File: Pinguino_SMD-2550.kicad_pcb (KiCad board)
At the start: 2 copper layers, 25.4 x 25.4 mm, 18 parts, among them P1 USB_OTG, P2 CONN_01X08, P3 CONN_01X02, P4 CONN_01X10, SW1 SW Reset, Y1 20Mhz

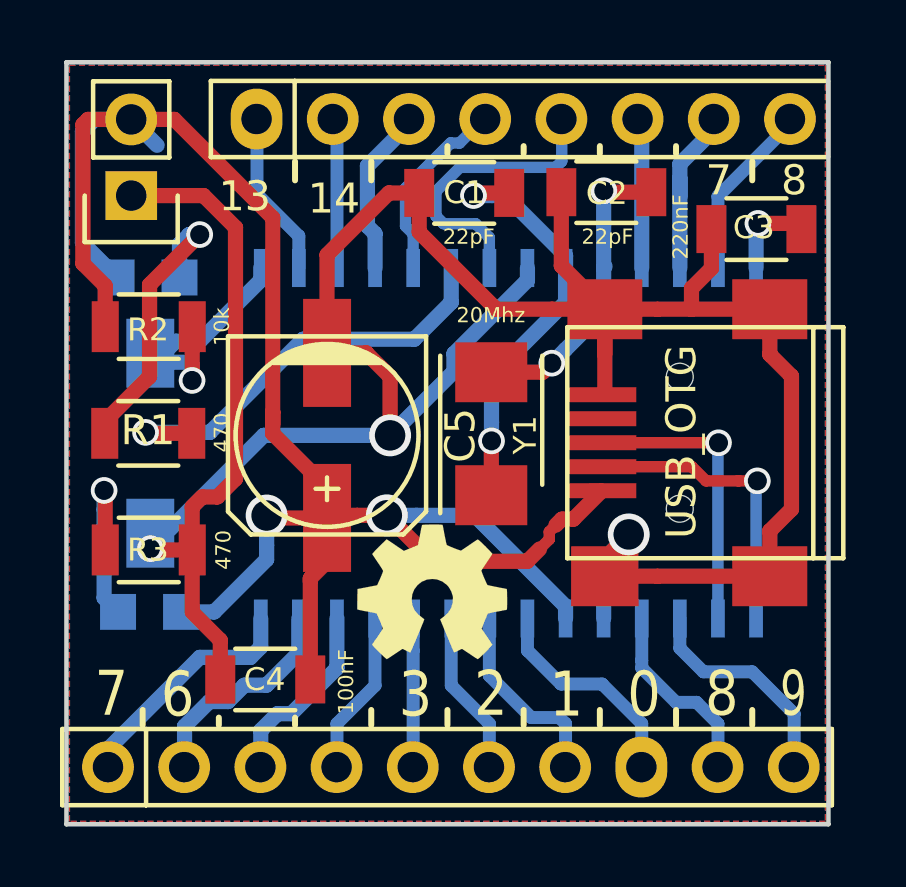
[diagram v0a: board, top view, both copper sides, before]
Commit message: F. SilkS
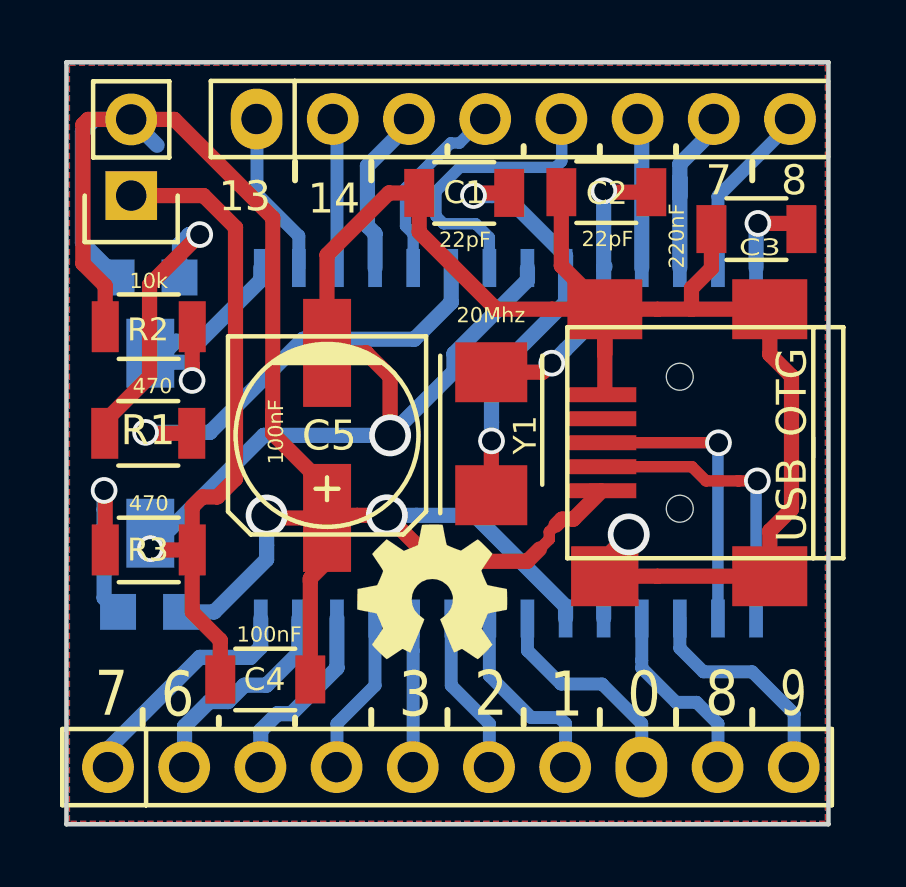
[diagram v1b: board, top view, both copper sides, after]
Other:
- board text added: "100nF"
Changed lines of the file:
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@@
-(kicad_pcb (version 4) (host pcbnew 4.0.2+dfsg1-2~bpo8+1-stable)
+(kicad_pcb (version 4) (host pcbnew 4.0.4+dfsg1-stable)
   (general
     (links 51)
     (no_connects 0)
-    (area 26.106 16.1873 57.158361 46.606001)
+    (area 21.689287 16.3373 57.158361 46.606001)
     (thickness 1.6)
-    (drawings 71)
+    (drawings 72)
     (tracks 278)
     (zones 0)
@@
     (visible_elements FFFFFF7F)
     (pcbplotparams
-      (layerselection 0x00000_80000001)
+      (layerselection 0x000f0_80000001)
       (usegerberextensions false)
       (excludeedgelayer true)
@@
       (effects (font (size 0.762 0.762) (thickness 0.127)))
     )
-    (fp_text value 22pF (at -0.1524 -1.4605 360) (layer F.SilkS)
+    (fp_text value 22pF (at -0.0254 -1.5621 360) (layer F.SilkS)
       (effects (font (size 0.508 0.508) (thickness 0.127)))
     )
@@
       (effects (font (size 0.762 0.762) (thickness 0.127)))
     )
-    (fp_text value 22pF (at 0.0381 1.4859) (layer F.SilkS)
+    (fp_text value 22pF (at 0.0381 1.5621) (layer F.SilkS)
       (effects (font (size 0.508 0.508) (thickness 0.127)))
     )
@@
     (tags "capacitor 1206")
     (attr smd)
-    (fp_text reference C3 (at 0.0889 0.0508 180) (layer F.SilkS)
-      (effects (font (size 0.762 0.762) (thickness 0.15)))
-    )
-    (fp_text value 220nF (at 2.5273 0.0762 450) (layer F.SilkS)
+    (fp_text reference C3 (at -0.1143 -0.6096 180) (layer F.SilkS)
+      (effects (font (size 0.56 0.762) (thickness 0.14)))
+    )
+    (fp_text value 220nF (at 2.6543 -0.2286 450) (layer F.SilkS)
       (effects (font (size 0.508 0.508) (thickness 0.125)))
     )
@@
       (effects (font (size 0.762 0.762) (thickness 0.127)))
     )
-    (fp_text value 100nF (at 2.6938 0.0762 90) (layer F.SilkS)
+    (fp_text value 100nF (at 0.1284 -1.4986 180) (layer F.SilkS)
       (effects (font (size 0.508 0.508) (thickness 0.127)))
     )
@@
       (effects (font (size 1 1) (thickness 0.15)))
     )
-    (fp_text value USB_OTG (at 0.79756 0.03302 270) (layer F.SilkS)
+    (fp_text value USB_OTG (at -2.88544 -0.06858 270) (layer F.SilkS)
       (effects (font (size 1 1) (thickness 0.15)))
     )
@@
       (effects (font (size 1 1) (thickness 0.15)))
     )
-    (fp_text value 470 (at 2.45364 -0.0254 90) (layer F.SilkS)
+    (fp_text value 470 (at 0.14224 -1.5748 180) (layer F.SilkS)
       (effects (font (size 0.508 0.508) (thickness 0.127)))
     )
@@
       (effects (font (size 0.762 0.762) (thickness 0.15)))
     )
-    (fp_text value 10k (at 2.4384 0 90) (layer F.SilkS)
+    (fp_text value 10k (at 0 -1.524 180) (layer F.SilkS)
       (effects (font (size 0.508 0.508) (thickness 0.127)))
     )
@@
       (effects (font (size 0.762 0.762) (thickness 0.15)))
     )
-    (fp_text value 470 (at 2.4892 0 90) (layer F.SilkS)
+    (fp_text value 470 (at 0 -1.5494 180) (layer F.SilkS)
       (effects (font (size 0.508 0.508) (thickness 0.1)))
     )
@@
     (descr "SMT capacitor, aluminium electrolytic, 6.3x5.3")
     (attr smd)
-    (fp_text reference C5 (at 0 -4.445 270) (layer F.SilkS)
+    (fp_text reference C5 (at 0.00762 -0.0762 360) (layer F.SilkS)
       (effects (font (size 1 1) (thickness 0.15)))
     )
@@
     )
   )
+  (gr_text 100nF (at 37.465 33.147 90) (layer F.SilkS)
+    (effects (font (size 0.508 0.508) (thickness 0.127)))
+  )
   (dimension 25.4 (width 0.3) (layer Dwgs.User)
     (gr_text "1,0000 in" (at 43.18 17.7) (layer Dwgs.User)
@@
     (effects (font (size 1.5 1.5) (thickness 0.3)) (justify mirror))
   )
-  (gr_text GND (at 34.544 25.654 90) (layer B.SilkS)
+  (gr_text GND (at 34.4424 25.4 90) (layer B.SilkS)
     (effects (font (size 0.8 0.8) (thickness 0.2)) (justify mirror))
   )
@@
     (effects (font (size 0.5 0.5) (thickness 0.125)) (justify mirror))
   )
-  (gr_text 16-RA3 (at 44.45 25.273 90) (layer B.SilkS)
+  (gr_text 16-RA3 (at 44.8056 25.2984 90) (layer B.SilkS)
     (effects (font (size 0.5 0.5) (thickness 0.125)) (justify mirror))
   )
